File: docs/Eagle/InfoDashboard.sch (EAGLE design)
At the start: 5 parts, among them X1 HD44780LCD-1602

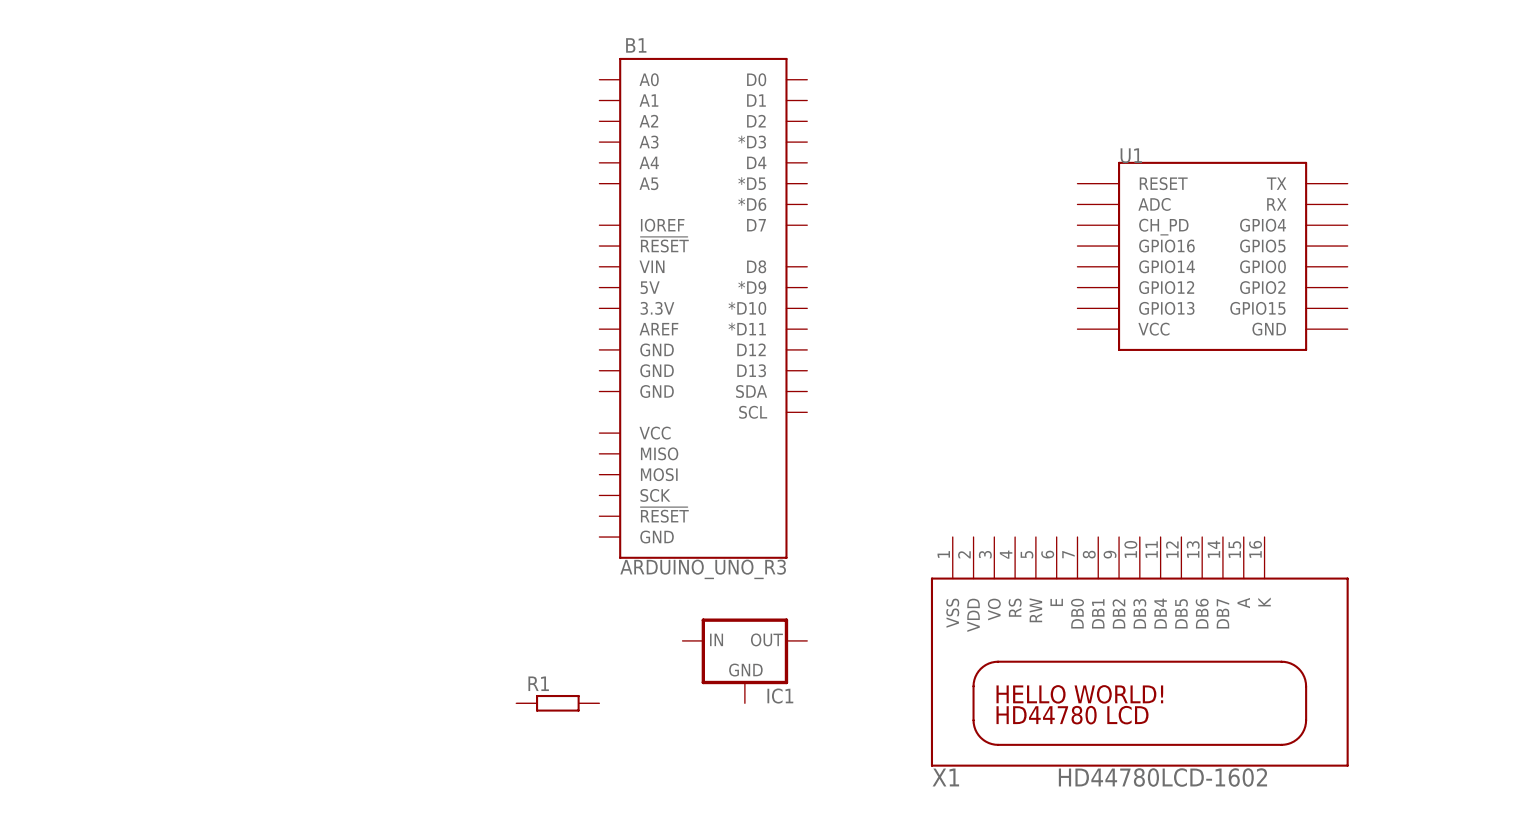
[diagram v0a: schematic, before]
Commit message: schematics finalized
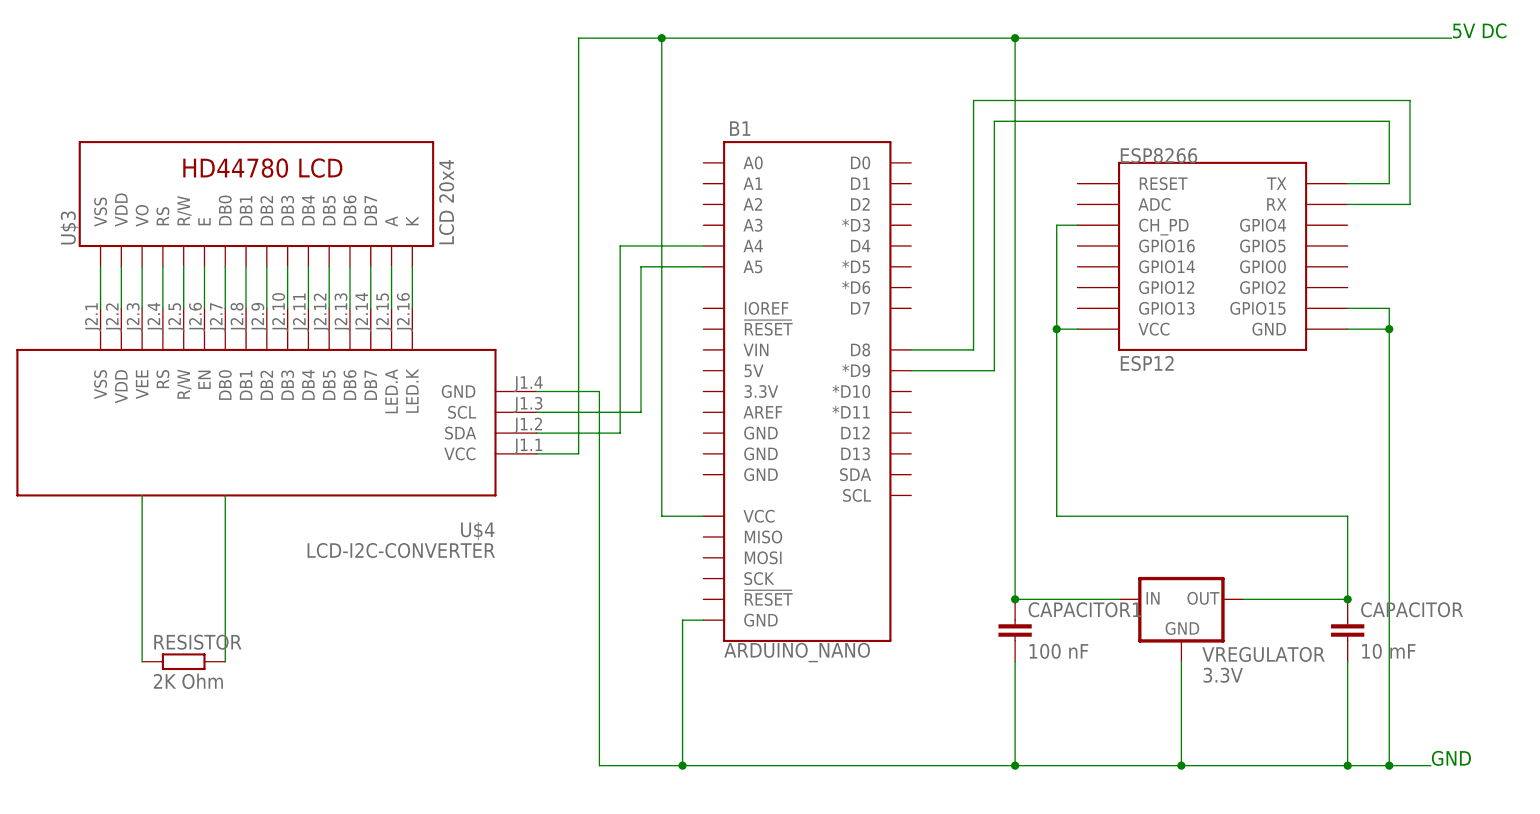
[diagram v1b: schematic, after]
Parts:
- removed IC1: (no value), DC_LOAD_AU:78LXX
- removed R1: (no value), eagle-ltspice:R
- removed X1: HD44780LCD-1602, adafruit:HD44780LCD-1602
- added CAPACITOR: 10 mF, Nordic_nRF:CAPACITOR_0201_L
- added CAPACITOR1: 100 nF, Nordic_nRF:CAPACITOR_0201_L
- added RESISTOR: 2K Ohm, eagle-ltspice:R
- added U$3: LCD 20x4, HD44780LCD2:LCD-HD4478016X2-4-HOLES-BL16X2-4-HOLES-BL
- added U$4: LCD-I2C-CONVERTER, diy-modules:LCD-I2C-CONVERTER
- added VREGULATOR: 3.3V, DC_LOAD_AU:78LXX
- B1: value ARDUINO_UNO_R3 -> ARDUINO_NANO
- ESP8266: value (none) -> ESP12
- renumbered U1 to ESP8266
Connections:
- new net N$1: B1.*D9, ESP8266.TX
- new net N$10: U$3.DB2, U$4.DB2
- new net N$11: U$3.DB3, U$4.DB3
- new net N$12: U$3.DB4, U$4.DB4
- new net N$13: U$3.DB5, U$4.DB5
- new net N$14: U$3.DB6, U$4.DB6
- new net N$15: U$3.DB7, U$4.DB7
- new net N$16: U$3.A, U$4.LED.A
- new net N$17: U$3.K, U$4.LED.K
- new net N$18: B1.A4, U$4.SDA
- new net N$19: B1.GND, CAPACITOR.2, CAPACITOR1.2, ESP8266.GND, ESP8266.GPIO15, U$4.GND, VREGULATOR.GND
- new net N$2: U$3.VSS, U$4.VSS
- new net N$20: B1.D8, B1.VCC, CAPACITOR1.1, ESP8266.RX, U$4.VCC, VREGULATOR.IN
- new net N$21: CAPACITOR.1, ESP8266.CH_PD, ESP8266.VCC, VREGULATOR.OUT
- new net N$22: B1.A5, U$4.SCL
- new net N$23: RESISTOR.1
- new net N$24: RESISTOR.2
- new net N$3: U$3.VDD, U$4.VDD
- new net N$4: U$3.VO, U$4.VEE
- new net N$5: U$3.RS, U$4.RS
- new net N$6: U$3.R/W, U$4.R/W
- new net N$7: U$3.E, U$4.EN
- new net N$8: U$3.DB0, U$4.DB0
- new net N$9: U$3.DB1, U$4.DB1
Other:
- note added: "5V DC"
- note added: "GND"
- moved on the sheet: B1
